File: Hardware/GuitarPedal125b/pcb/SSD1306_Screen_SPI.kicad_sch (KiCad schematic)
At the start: 1 part, among them U6 OLED_DISPLAY_SSD1306_SPI

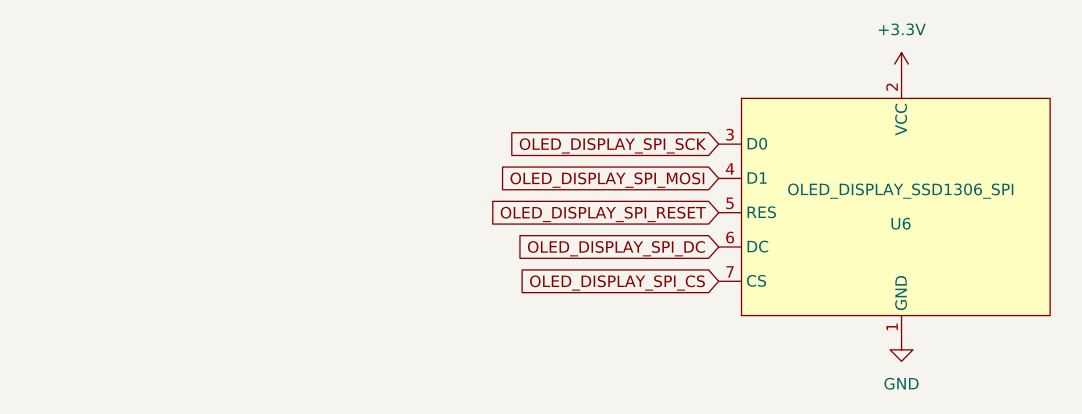
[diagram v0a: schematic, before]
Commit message: Continuing to work on Rev 6
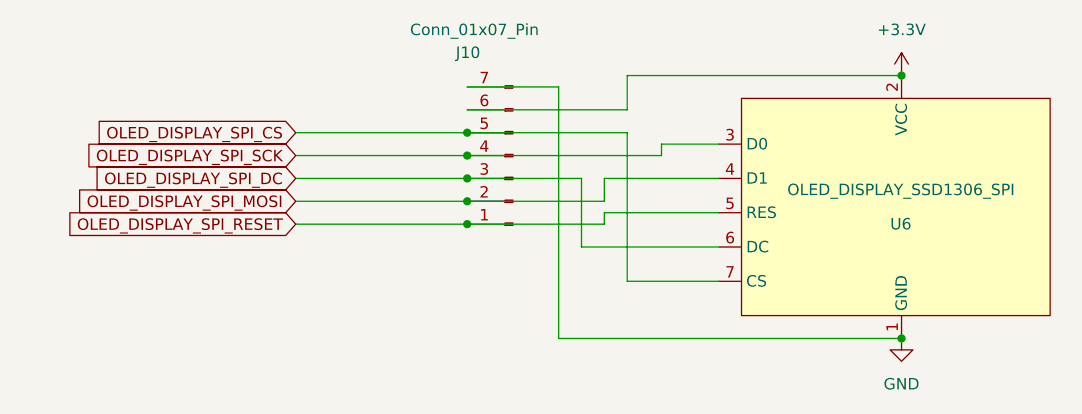
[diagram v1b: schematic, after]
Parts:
- added J10: Conn_01x07_Pin, Connector_Molex:Molex_PicoBlade_53398-0771_1x07-1MP_P1.25mm_Vertical, symbol Connector:Conn_01x07_Pin
- U6: footprint GuitarPedal125B:HiLetgo_OLED_SPI -> GuitarPedal125B:HiLetgo_OLED_SPI_NOPINS
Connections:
- net +3.3V: now also J10.6 (Pin_6)
- net GND: now also J10.7 (Pin_7)
- net OLED_DISPLAY_SPI_CS: now also J10.5 (Pin_5)
- net OLED_DISPLAY_SPI_DC: now also J10.3 (Pin_3)
- net OLED_DISPLAY_SPI_MOSI: now also J10.2 (Pin_2)
- net OLED_DISPLAY_SPI_RESET: now also J10.1 (Pin_1)
- net OLED_DISPLAY_SPI_SCK: now also J10.4 (Pin_4)
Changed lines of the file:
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@@
     (company "Made by Keith Shepherd (kshep@mac.com)")
   )
-  (global_label "OLED_DISPLAY_SPI_RESET" (shape input) (at 118.11 99.06 180) (fields_autoplaced)
-    (effects (font (size 1.27 1.27)) (justify right))
-    (property "Intersheetrefs" "${INTERSHEET_REFS}" (at 91.6274 98.9806 0)
-      (effects (font (size 1.27 1.27)) (justify right) hide)
-    )
-  )
-  (global_label "OLED_DISPLAY_SPI_CS" (shape input) (at 118.11 106.68 180) (fields_autoplaced)
-    (effects (font (size 1.27 1.27)) (justify right))
-    (property "Intersheetrefs" "${INTERSHEET_REFS}" (at 94.8931 106.6006 0)
-      (effects (font (size 1.27 1.27)) (justify right) hide)
-    )
-  )
-  (global_label "OLED_DISPLAY_SPI_DC" (shape input) (at 118.11 102.87 180) (fields_autoplaced)
-    (effects (font (size 1.27 1.27)) (justify right))
-    (property "Intersheetrefs" "${INTERSHEET_REFS}" (at 94.8326 102.7906 0)
-      (effects (font (size 1.27 1.27)) (justify right) hide)
-    )
-  )
-  (global_label "OLED_DISPLAY_SPI_MOSI" (shape input) (at 118.11 95.25 180) (fields_autoplaced)
-    (effects (font (size 1.27 1.27)) (justify right))
-    (property "Intersheetrefs" "${INTERSHEET_REFS}" (at 92.7764 95.1706 0)
-      (effects (font (size 1.27 1.27)) (justify right) hide)
-    )
-  )
-  (global_label "OLED_DISPLAY_SPI_SCK" (shape input) (at 118.11 91.44 180) (fields_autoplaced)
-    (effects (font (size 1.27 1.27)) (justify right))
-    (property "Intersheetrefs" "${INTERSHEET_REFS}" (at 93.6231 91.3606 0)
-      (effects (font (size 1.27 1.27)) (justify right) hide)
+  (junction (at 90.17 100.33) (diameter 0) (color 0 0 0 0)
+  )
+  (junction (at 138.43 113.03) (diameter 0) (color 0 0 0 0)
+  )
+  (junction (at 90.17 95.25) (diameter 0) (color 0 0 0 0)
+  )
+  (junction (at 138.43 83.82) (diameter 0) (color 0 0 0 0)
+  )
+  (junction (at 90.17 90.17) (diameter 0) (color 0 0 0 0)
+  )
+  (junction (at 90.17 92.71) (diameter 0) (color 0 0 0 0)
+  )
+  (junction (at 90.17 97.79) (diameter 0) (color 0 0 0 0)
+  )
+  (wire (pts (xy 90.17 87.63) (xy 107.95 87.63))
+    (stroke (width 0) (type default))
+  )
+  (wire (pts (xy 90.17 100.33) (xy 105.41 100.33))
+    (stroke (width 0) (type default))
+  )
+  (wire (pts (xy 105.41 99.06) (xy 118.11 99.06))
+    (stroke (width 0) (type default))
+  )
+  (wire (pts (xy 105.41 97.79) (xy 105.41 95.25))
+    (stroke (width 0) (type default))
+  )
+  (wire (pts (xy 105.41 95.25) (xy 118.11 95.25))
+    (stroke (width 0) (type default))
+  )
+  (wire (pts (xy 100.33 113.03) (xy 138.43 113.03))
+    (stroke (width 0) (type default))
+  )
+  (wire (pts (xy 102.87 95.25) (xy 102.87 102.87))
+    (stroke (width 0) (type default))
+  )
+  (wire (pts (xy 71.12 100.33) (xy 90.17 100.33))
+    (stroke (width 0) (type default))
+  )
+  (wire (pts (xy 102.87 102.87) (xy 118.11 102.87))
+    (stroke (width 0) (type default))
+  )
+  (wire (pts (xy 107.95 90.17) (xy 107.95 106.68))
+    (stroke (width 0) (type default))
+  )
+  (wire (pts (xy 111.76 91.44) (xy 118.11 91.44))
+    (stroke (width 0) (type default))
+  )
+  (wire (pts (xy 105.41 100.33) (xy 105.41 99.06))
+    (stroke (width 0) (type default))
+  )
+  (wire (pts (xy 90.17 95.25) (xy 102.87 95.25))
+    (stroke (width 0) (type default))
+  )
+  (wire (pts (xy 90.17 97.79) (xy 105.41 97.79))
+    (stroke (width 0) (type default))
+  )
+  (wire (pts (xy 107.95 83.82) (xy 138.43 83.82))
+    (stroke (width 0) (type default))
+  )
+  (wire (pts (xy 90.17 85.09) (xy 100.33 85.09))
+    (stroke (width 0) (type default))
+  )
+  (wire (pts (xy 90.17 92.71) (xy 111.76 92.71))
+    (stroke (width 0) (type default))
+  )
+  (wire (pts (xy 71.12 92.71) (xy 90.17 92.71))
+    (stroke (width 0) (type default))
+  )
+  (wire (pts (xy 71.12 90.17) (xy 90.17 90.17))
+    (stroke (width 0) (type default))
+  )
+  (wire (pts (xy 107.95 106.68) (xy 118.11 106.68))
+    (stroke (width 0) (type default))
+  )
+  (wire (pts (xy 71.12 95.25) (xy 90.17 95.25))
+    (stroke (width 0) (type default))
+  )
+  (wire (pts (xy 111.76 92.71) (xy 111.76 91.44))
+    (stroke (width 0) (type default))
+  )
+  (wire (pts (xy 90.17 90.17) (xy 107.95 90.17))
+    (stroke (width 0) (type default))
+  )
+  (wire (pts (xy 100.33 85.09) (xy 100.33 113.03))
+    (stroke (width 0) (type default))
+  )
+  (wire (pts (xy 71.12 97.79) (xy 90.17 97.79))
+    (stroke (width 0) (type default))
+  )
+  (wire (pts (xy 107.95 87.63) (xy 107.95 83.82))
+    (stroke (width 0) (type default))
+  )
+  (global_label "OLED_DISPLAY_SPI_RESET" (shape input) (at 71.12 100.33 180) (fields_autoplaced)
+    (effects (font (size 1.27 1.27)) (justify right))
+    (property "Intersheetrefs" "${INTERSHEET_REFS}" (at 44.6374 100.2506 0)
+      (effects (font (size 1.27 1.27)) (justify right) hide)
+    )
+  )
+  (global_label "OLED_DISPLAY_SPI_CS" (shape input) (at 71.12 90.17 180) (fields_autoplaced)
+    (effects (font (size 1.27 1.27)) (justify right))
+    (property "Intersheetrefs" "${INTERSHEET_REFS}" (at 47.9031 90.0906 0)
+      (effects (font (size 1.27 1.27)) (justify right) hide)
+    )
+  )
+  (global_label "OLED_DISPLAY_SPI_DC" (shape input) (at 71.12 95.25 180) (fields_autoplaced)
+    (effects (font (size 1.27 1.27)) (justify right))
+    (property "Intersheetrefs" "${INTERSHEET_REFS}" (at 47.8426 95.1706 0)
+      (effects (font (size 1.27 1.27)) (justify right) hide)
+    )
+  )
+  (global_label "OLED_DISPLAY_SPI_MOSI" (shape input) (at 71.12 97.79 180) (fields_autoplaced)
+    (effects (font (size 1.27 1.27)) (justify right))
+    (property "Intersheetrefs" "${INTERSHEET_REFS}" (at 45.7864 97.7106 0)
+      (effects (font (size 1.27 1.27)) (justify right) hide)
+    )
+  )
+  (global_label "OLED_DISPLAY_SPI_SCK" (shape input) (at 71.12 92.71 180) (fields_autoplaced)
+    (effects (font (size 1.27 1.27)) (justify right))
+    (property "Intersheetrefs" "${INTERSHEET_REFS}" (at 46.6331 92.6306 0)
+      (effects (font (size 1.27 1.27)) (justify right) hide)
+    )
+  )
+  (symbol (lib_id "Connector:Conn_01x07_Pin") (at 95.25 92.71 180) (unit 1)
+    (in_bom yes) (on_board yes) (dnp no)
+    (property "Reference" "J10" (at 88.9 81.28 0)
+      (effects (font (size 1.27 1.27)) (justify right))
+    )
+    (property "Value" "Conn_01x07_Pin" (at 83.82 78.74 0)
+      (effects (font (size 1.27 1.27)) (justify right))
+    )
+    (property "Footprint" "Connector_Molex:Molex_PicoBlade_53398-0771_1x07-1MP_P1.25mm_Vertical" (at 95.25 92.71 0)
+      (effects (font (size 1.27 1.27)) hide)
+    )
+    (property "Datasheet" "~" (at 95.25 92.71 0)
+      (effects (font (size 1.27 1.27)) hide)
+    )
+    (pin "5")
+    (pin "1")
+    (pin "2")
+    (pin "3")
+    (pin "4")
+    (pin "7")
+    (pin "6")
+    (instances
+      (project "DaisySeedPedal125b"
+        (path "/1d54e6f4-7c7a-4f03-b2db-a136bdff5b99/05a79108-cb22-4356-96de-706d080a4feb"
+          (reference "J10") (unit 1)
+        )
+      )
     )
   )
   (symbol (lib_id "power:GND") (at 138.43 113.03 0) (unit 1)
     (in_bom yes) (on_board yes) (dnp no) (fields_autoplaced)
-    (property "Reference" "#PWR08" (at 138.43 119.38 0)
+    (property "Reference" "#PWR063" (at 138.43 119.38 0)
       (effects (font (size 1.27 1.27)) hide)
     )
@@
       (project "DaisySeedPedal125b"
         (path "/1d54e6f4-7c7a-4f03-b2db-a136bdff5b99/05a79108-cb22-4356-96de-706d080a4feb"
-          (reference "#PWR08") (unit 1)
+          (reference "#PWR063") (unit 1)
         )
       )
@@
       (effects (font (size 1.27 1.27)) (justify left))
     )
-    (property "Footprint" "GuitarPedal125B:HiLetgo_OLED_SPI" (at 138.43 102.87 0)
+    (property "Footprint" "GuitarPedal125B:HiLetgo_OLED_SPI_NOPINS" (at 138.43 102.87 0)
       (effects (font (size 1.27 1.27)) hide)
     )
@@
   (symbol (lib_id "power:+3.3V") (at 138.43 83.82 0) (unit 1)
     (in_bom yes) (on_board yes) (dnp no) (fields_autoplaced)
-    (property "Reference" "#PWR01" (at 138.43 87.63 0)
+    (property "Reference" "#PWR064" (at 138.43 87.63 0)
       (effects (font (size 1.27 1.27)) hide)
     )
@@
       (project "DaisySeedPedal125b"
         (path "/1d54e6f4-7c7a-4f03-b2db-a136bdff5b99/05a79108-cb22-4356-96de-706d080a4feb"
-          (reference "#PWR01") (unit 1)
-        )
-      )
+          (reference "#PWR064") (unit 1)
+        )
+      )

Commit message: More work on layout
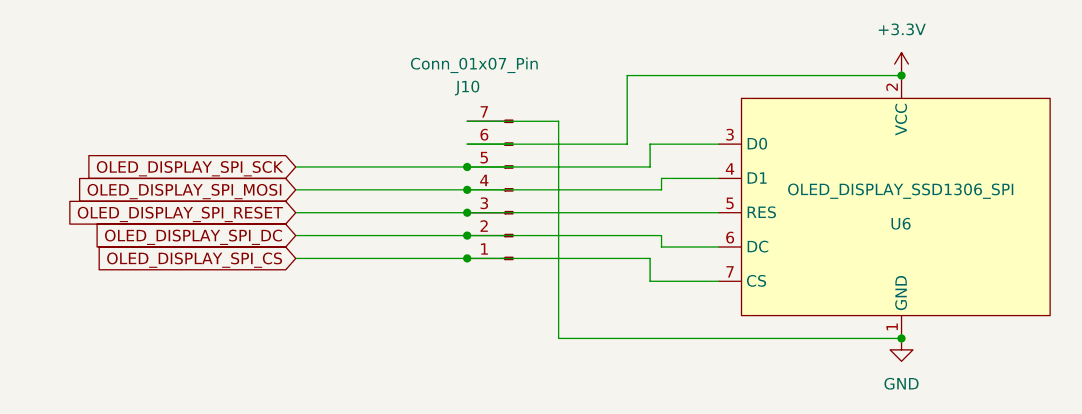
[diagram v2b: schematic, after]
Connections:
- net OLED_DISPLAY_SPI_CS: now also J10.1 (Pin_1); no longer J10.5 (Pin_5)
- net OLED_DISPLAY_SPI_DC: now also J10.2 (Pin_2); no longer J10.3 (Pin_3)
- net OLED_DISPLAY_SPI_MOSI: now also J10.4 (Pin_4); no longer J10.2 (Pin_2)
- net OLED_DISPLAY_SPI_RESET: now also J10.3 (Pin_3); no longer J10.1 (Pin_1)
- net OLED_DISPLAY_SPI_SCK: now also J10.5 (Pin_5); no longer J10.4 (Pin_4)
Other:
- moved on the sheet: J10
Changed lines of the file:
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@@
     (company "Made by Keith Shepherd (kshep@mac.com)")
   )
-  (junction (at 90.17 100.33) (diameter 0) (color 0 0 0 0)
+  (junction (at 90.17 96.52) (diameter 0) (color 0 0 0 0)
+  )
+  (junction (at 90.17 101.6) (diameter 0) (color 0 0 0 0)
   )
   (junction (at 138.43 113.03) (diameter 0) (color 0 0 0 0)
   )
-  (junction (at 90.17 95.25) (diameter 0) (color 0 0 0 0)
+  (junction (at 90.17 93.98) (diameter 0) (color 0 0 0 0)
+  )
+  (junction (at 90.17 99.06) (diameter 0) (color 0 0 0 0)
   )
   (junction (at 138.43 83.82) (diameter 0) (color 0 0 0 0)
   )
-  (junction (at 90.17 90.17) (diameter 0) (color 0 0 0 0)
+  (junction (at 90.17 104.14) (diameter 0) (color 0 0 0 0)
   )
-  (junction (at 90.17 92.71) (diameter 0) (color 0 0 0 0)
-  )
-  (junction (at 90.17 97.79) (diameter 0) (color 0 0 0 0)
-  )
-  (wire (pts (xy 90.17 87.63) (xy 107.95 87.63))
+  (wire (pts (xy 90.17 91.44) (xy 107.95 91.44))
     (stroke (width 0) (type default))
   )
-  (wire (pts (xy 90.17 100.33) (xy 105.41 100.33))
+  (wire (pts (xy 111.76 101.6) (xy 111.76 102.87))
     (stroke (width 0) (type default))
   )
-  (wire (pts (xy 105.41 99.06) (xy 118.11 99.06))
+  (wire (pts (xy 110.49 91.44) (xy 118.11 91.44))
     (stroke (width 0) (type default))
   )
-  (wire (pts (xy 105.41 97.79) (xy 105.41 95.25))
+  (wire (pts (xy 110.49 93.98) (xy 110.49 91.44))
     (stroke (width 0) (type default))
   )
-  (wire (pts (xy 105.41 95.25) (xy 118.11 95.25))
+  (wire (pts (xy 111.76 96.52) (xy 111.76 95.25))
+    (stroke (width 0) (type default))
+  )
+  (wire (pts (xy 90.17 104.14) (xy 110.49 104.14))
+    (stroke (width 0) (type default))
+  )
+  (wire (pts (xy 118.11 106.68) (xy 110.49 106.68))
+    (stroke (width 0) (type default))
+  )
+  (wire (pts (xy 110.49 106.68) (xy 110.49 104.14))
     (stroke (width 0) (type default))
   )
@@
     (stroke (width 0) (type default))
   )
-  (wire (pts (xy 102.87 95.25) (xy 102.87 102.87))
+  (wire (pts (xy 71.12 104.14) (xy 90.17 104.14))
     (stroke (width 0) (type default))
   )
-  (wire (pts (xy 71.12 100.33) (xy 90.17 100.33))
-    (stroke (width 0) (type default))
-  )
-  (wire (pts (xy 102.87 102.87) (xy 118.11 102.87))
-    (stroke (width 0) (type default))
-  )
-  (wire (pts (xy 107.95 90.17) (xy 107.95 106.68))
-    (stroke (width 0) (type default))
-  )
-  (wire (pts (xy 111.76 91.44) (xy 118.11 91.44))
-    (stroke (width 0) (type default))
-  )
-  (wire (pts (xy 105.41 100.33) (xy 105.41 99.06))
-    (stroke (width 0) (type default))
-  )
-  (wire (pts (xy 90.17 95.25) (xy 102.87 95.25))
-    (stroke (width 0) (type default))
-  )
-  (wire (pts (xy 90.17 97.79) (xy 105.41 97.79))
+  (wire (pts (xy 90.17 99.06) (xy 118.11 99.06))
     (stroke (width 0) (type default))
   )
@@
     (stroke (width 0) (type default))
   )
-  (wire (pts (xy 90.17 85.09) (xy 100.33 85.09))
+  (wire (pts (xy 90.17 88.9) (xy 100.33 88.9))
     (stroke (width 0) (type default))
   )
-  (wire (pts (xy 90.17 92.71) (xy 111.76 92.71))
+  (wire (pts (xy 111.76 96.52) (xy 90.17 96.52))
     (stroke (width 0) (type default))
   )
-  (wire (pts (xy 71.12 92.71) (xy 90.17 92.71))
+  (wire (pts (xy 71.12 96.52) (xy 90.17 96.52))
     (stroke (width 0) (type default))
   )
-  (wire (pts (xy 71.12 90.17) (xy 90.17 90.17))
+  (wire (pts (xy 71.12 93.98) (xy 90.17 93.98))
     (stroke (width 0) (type default))
   )
-  (wire (pts (xy 107.95 106.68) (xy 118.11 106.68))
+  (wire (pts (xy 71.12 99.06) (xy 90.17 99.06))
     (stroke (width 0) (type default))
   )
-  (wire (pts (xy 71.12 95.25) (xy 90.17 95.25))
+  (wire (pts (xy 111.76 101.6) (xy 90.17 101.6))
     (stroke (width 0) (type default))
   )
-  (wire (pts (xy 111.76 92.71) (xy 111.76 91.44))
+  (wire (pts (xy 90.17 93.98) (xy 110.49 93.98))
     (stroke (width 0) (type default))
   )
-  (wire (pts (xy 90.17 90.17) (xy 107.95 90.17))
+  (wire (pts (xy 118.11 95.25) (xy 111.76 95.25))
     (stroke (width 0) (type default))
   )
-  (wire (pts (xy 100.33 85.09) (xy 100.33 113.03))
+  (wire (pts (xy 100.33 88.9) (xy 100.33 113.03))
     (stroke (width 0) (type default))
   )
-  (wire (pts (xy 71.12 97.79) (xy 90.17 97.79))
+  (wire (pts (xy 71.12 101.6) (xy 90.17 101.6))
     (stroke (width 0) (type default))
   )
-  (wire (pts (xy 107.95 87.63) (xy 107.95 83.82))
+  (wire (pts (xy 118.11 102.87) (xy 111.76 102.87))
     (stroke (width 0) (type default))
   )
-  (global_label "OLED_DISPLAY_SPI_RESET" (shape input) (at 71.12 100.33 180) (fields_autoplaced)
+  (wire (pts (xy 107.95 91.44) (xy 107.95 83.82))
+    (stroke (width 0) (type default))
+  )
+  (global_label "OLED_DISPLAY_SPI_RESET" (shape input) (at 71.12 99.06 180) (fields_autoplaced)
     (effects (font (size 1.27 1.27)) (justify right))
-    (property "Intersheetrefs" "${INTERSHEET_REFS}" (at 44.6374 100.2506 0)
+    (property "Intersheetrefs" "${INTERSHEET_REFS}" (at 44.6374 98.9806 0)
       (effects (font (size 1.27 1.27)) (justify right) hide)
     )
   )
-  (global_label "OLED_DISPLAY_SPI_CS" (shape input) (at 71.12 90.17 180) (fields_autoplaced)
+  (global_label "OLED_DISPLAY_SPI_CS" (shape input) (at 71.12 104.14 180) (fields_autoplaced)
     (effects (font (size 1.27 1.27)) (justify right))
-    (property "Intersheetrefs" "${INTERSHEET_REFS}" (at 47.9031 90.0906 0)
+    (property "Intersheetrefs" "${INTERSHEET_REFS}" (at 47.9031 104.0606 0)
       (effects (font (size 1.27 1.27)) (justify right) hide)
     )
   )
-  (global_label "OLED_DISPLAY_SPI_DC" (shape input) (at 71.12 95.25 180) (fields_autoplaced)
+  (global_label "OLED_DISPLAY_SPI_DC" (shape input) (at 71.12 101.6 180) (fields_autoplaced)
     (effects (font (size 1.27 1.27)) (justify right))
-    (property "Intersheetrefs" "${INTERSHEET_REFS}" (at 47.8426 95.1706 0)
+    (property "Intersheetrefs" "${INTERSHEET_REFS}" (at 47.8426 101.5206 0)
       (effects (font (size 1.27 1.27)) (justify right) hide)
     )
   )
-  (global_label "OLED_DISPLAY_SPI_MOSI" (shape input) (at 71.12 97.79 180) (fields_autoplaced)
+  (global_label "OLED_DISPLAY_SPI_MOSI" (shape input) (at 71.12 96.52 180) (fields_autoplaced)
     (effects (font (size 1.27 1.27)) (justify right))
-    (property "Intersheetrefs" "${INTERSHEET_REFS}" (at 45.7864 97.7106 0)
+    (property "Intersheetrefs" "${INTERSHEET_REFS}" (at 45.7864 96.4406 0)
       (effects (font (size 1.27 1.27)) (justify right) hide)
     )
   )
-  (global_label "OLED_DISPLAY_SPI_SCK" (shape input) (at 71.12 92.71 180) (fields_autoplaced)
+  (global_label "OLED_DISPLAY_SPI_SCK" (shape input) (at 71.12 93.98 180) (fields_autoplaced)
     (effects (font (size 1.27 1.27)) (justify right))
-    (property "Intersheetrefs" "${INTERSHEET_REFS}" (at 46.6331 92.6306 0)
+    (property "Intersheetrefs" "${INTERSHEET_REFS}" (at 46.6331 93.9006 0)
       (effects (font (size 1.27 1.27)) (justify right) hide)
     )
   )
-  (symbol (lib_id "Connector:Conn_01x07_Pin") (at 95.25 92.71 180) (unit 1)
+  (symbol (lib_id "Connector:Conn_01x07_Pin") (at 95.25 96.52 180) (unit 1)
     (in_bom yes) (on_board yes) (dnp no)
-    (property "Reference" "J10" (at 88.9 81.28 0)
+    (property "Reference" "J10" (at 88.9 85.09 0)
       (effects (font (size 1.27 1.27)) (justify right))
     )
-    (property "Value" "Conn_01x07_Pin" (at 83.82 78.74 0)
+    (property "Value" "Conn_01x07_Pin" (at 83.82 82.55 0)
       (effects (font (size 1.27 1.27)) (justify right))
     )
-    (property "Footprint" "Connector_Molex:Molex_PicoBlade_53398-0771_1x07-1MP_P1.25mm_Vertical" (at 95.25 92.71 0)
+    (property "Footprint" "Connector_Molex:Molex_PicoBlade_53398-0771_1x07-1MP_P1.25mm_Vertical" (at 95.25 96.52 0)
       (effects (font (size 1.27 1.27)) hide)
     )
-    (property "Datasheet" "~" (at 95.25 92.71 0)
+    (property "Datasheet" "~" (at 95.25 96.52 0)
       (effects (font (size 1.27 1.27)) hide)
     )
